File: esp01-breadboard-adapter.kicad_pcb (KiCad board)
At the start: 2 copper layers, 3 parts, among them P1 CONN_02X04, P2 CONN_01X04, P3 CONN_01X04

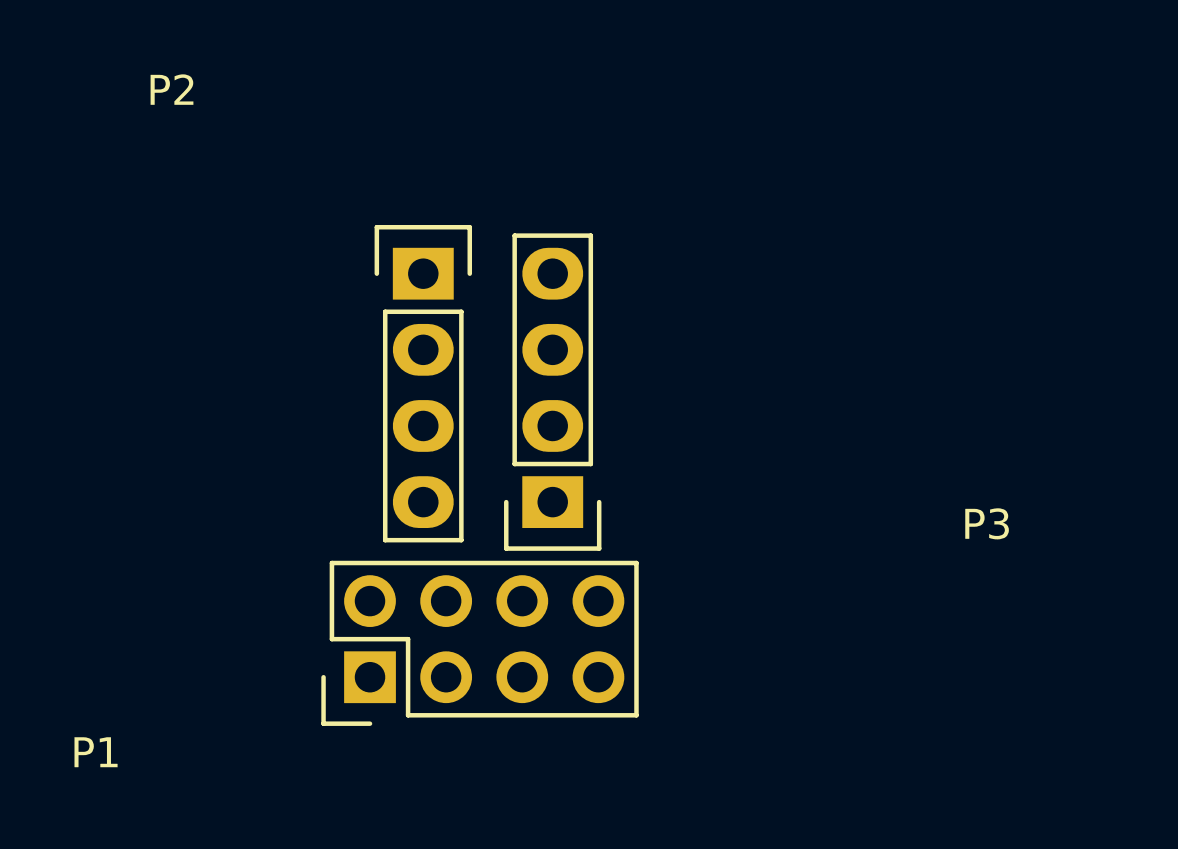
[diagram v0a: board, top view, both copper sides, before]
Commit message: begin 2nd layer pcb
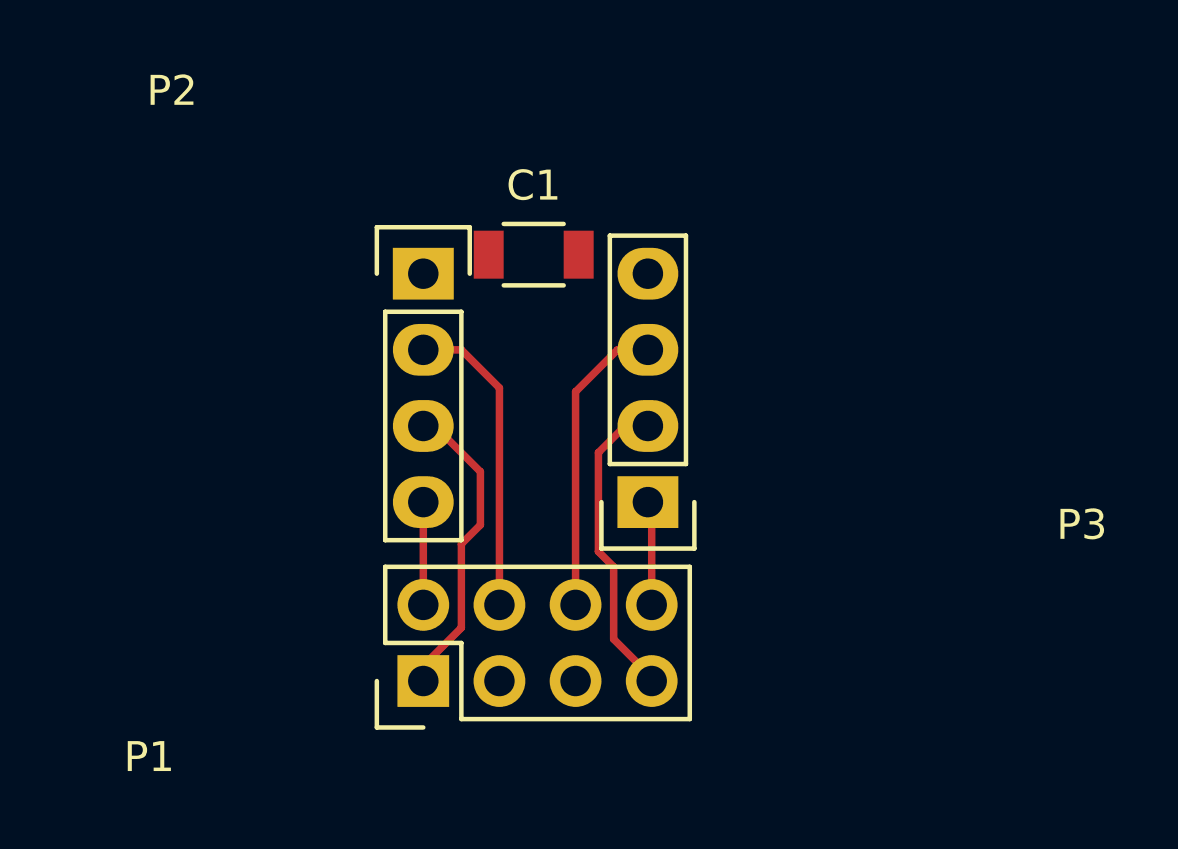
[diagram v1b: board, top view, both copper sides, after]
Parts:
- added C1: C, Capacitors_SMD:C_1206, F.Cu at (137.0, 106.6)
- moved P3 3.17 mm to (140.8, 114.8)
- moved P1 1.78 mm to (133.3, 120.8)
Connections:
- P2 pad 1: RXD -> GPIO0
- P2 pad 2: GPIO0 -> RESET
- P2 pad 3: GPIO2 -> RXD
- P2 pad 4: GND -> VCC
- P3 pad 2: CH_PD -> GND
- P3 pad 3: RESET -> CH_PD
- P3 pad 4: VCC -> GPIO2
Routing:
- net GND: track 0.00 -> 10.4 mm
- net RXD: track 0.00 -> 10.3 mm
- net RESET: track 0.00 -> 10.3 mm
- net CH_PD: track 0.00 -> 10.1 mm
- net TXD: track 0.00 -> 3.48 mm
- net VCC: track 0.00 -> 3.43 mm
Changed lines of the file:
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@@
 (kicad_pcb (version 4) (host pcbnew 4.0.2-stable)
   (general
-    (links 8)
-    (no_connects 8)
+    (links 10)
+    (no_connects 4)
     (area 0 0 0 0)
     (thickness 1.6)
     (drawings 0)
-    (tracks 0)
+    (tracks 23)
     (zones 0)
-    (modules 3)
+    (modules 4)
     (nets 9)
   )
@@
     (pad_to_mask_clearance 0.2)
     (aux_axis_origin 0 0)
-    (visible_elements FFFFFF7F)
+    (visible_elements 7FFFFFFF)
     (pcbplotparams
       (layerselection 0x00030_80000001)
@@
   )
   (module Pin_Headers:Pin_Header_Straight_2x04 (layer F.Cu)
-    (at 131.572 120.65 90)
+    (at 133.35 120.777 90)
     (descr "Through hole pin header")
     (tags "pin header")
@@
     (fp_line (start -1.55 -1.55) (end 1.55 -1.55) (layer F.SilkS) (width 0.15))
     (pad 1 thru_hole rect (at 0 0) (size 2.032 1.7272) (drill 1.016) (layers *.Cu *.Mask)
+      (net 3 GPIO0))
+    (pad 2 thru_hole oval (at 0 2.54) (size 2.032 1.7272) (drill 1.016) (layers *.Cu *.Mask)
+      (net 4 RESET))
+    (pad 3 thru_hole oval (at 0 5.08) (size 2.032 1.7272) (drill 1.016) (layers *.Cu *.Mask)
       (net 1 RXD))
-    (pad 2 thru_hole oval (at 0 2.54) (size 2.032 1.7272) (drill 1.016) (layers *.Cu *.Mask)
-      (net 3 GPIO0))
-    (pad 3 thru_hole oval (at 0 5.08) (size 2.032 1.7272) (drill 1.016) (layers *.Cu *.Mask)
-      (net 5 GPIO2))
     (pad 4 thru_hole oval (at 0 7.62) (size 2.032 1.7272) (drill 1.016) (layers *.Cu *.Mask)
-      (net 7 GND))
+      (net 2 VCC))
     (model Pin_Headers.3dshapes/Pin_Header_Straight_1x04.wrl
       (at (xyz 0 -0.15 0))
@@
   )
   (module Pin_Headers:Pin_Header_Straight_1x04 (layer F.Cu)
-    (at 137.668 114.808 180)
+    (at 140.843 114.808 180)
     (descr "Through hole pin header")
     (tags "pin header")
@@
       (net 8 TXD))
     (pad 2 thru_hole oval (at 0 2.54 180) (size 2.032 1.7272) (drill 1.016) (layers *.Cu *.Mask)
+      (net 7 GND))
+    (pad 3 thru_hole oval (at 0 5.08 180) (size 2.032 1.7272) (drill 1.016) (layers *.Cu *.Mask)
       (net 6 CH_PD))
-    (pad 3 thru_hole oval (at 0 5.08 180) (size 2.032 1.7272) (drill 1.016) (layers *.Cu *.Mask)
-      (net 4 RESET))
     (pad 4 thru_hole oval (at 0 7.62 180) (size 2.032 1.7272) (drill 1.016) (layers *.Cu *.Mask)
-      (net 2 VCC))
+      (net 5 GPIO2))
     (model Pin_Headers.3dshapes/Pin_Header_Straight_1x04.wrl
       (at (xyz 0 -0.15 0))
@@
     )
   )
+  (module Capacitors_SMD:C_1206 (layer F.Cu)
+    (at 137.033 106.553)
+    (descr "Capacitor SMD 1206, reflow soldering, AVX (see smccp.pdf)")
+    (tags "capacitor 1206")
+    (attr smd)
+    (fp_text reference C1 (at 0 -2.3) (layer F.SilkS)
+      (effects (font (size 1 1) (thickness 0.15)))
+    )
+    (fp_text value C (at 0 2.3) (layer F.Fab)
+      (effects (font (size 1 1) (thickness 0.15)))
+    )
+    (fp_line (start -1.6 0.8) (end -1.6 -0.8) (layer F.Fab) (width 0.15))
+    (fp_line (start 1.6 0.8) (end -1.6 0.8) (layer F.Fab) (width 0.15))
+    (fp_line (start 1.6 -0.8) (end 1.6 0.8) (layer F.Fab) (width 0.15))
+    (fp_line (start -1.6 -0.8) (end 1.6 -0.8) (layer F.Fab) (width 0.15))
+    (fp_line (start -2.3 -1.15) (end 2.3 -1.15) (layer F.CrtYd) (width 0.05))
+    (fp_line (start -2.3 1.15) (end 2.3 1.15) (layer F.CrtYd) (width 0.05))
+    (fp_line (start -2.3 -1.15) (end -2.3 1.15) (layer F.CrtYd) (width 0.05))
+    (fp_line (start 2.3 -1.15) (end 2.3 1.15) (layer F.CrtYd) (width 0.05))
+    (fp_line (start 1 -1.025) (end -1 -1.025) (layer F.SilkS) (width 0.15))
+    (fp_line (start -1 1.025) (end 1 1.025) (layer F.SilkS) (width 0.15))
+    (pad 1 smd rect (at -1.5 0) (size 1 1.6) (layers F.Cu F.Paste F.Mask)
+      (net 2 VCC))
+    (pad 2 smd rect (at 1.5 0) (size 1 1.6) (layers F.Cu F.Paste F.Mask)
+      (net 7 GND))
+    (model Capacitors_SMD.3dshapes/C_1206.wrl
+      (at (xyz 0 0 0))
+      (scale (xyz 1 1 1))
+      (rotate (xyz 0 0 0))
+    )
+  )
+  (segment (start 133.35 120.777) (end 133.35 120.269) (width 0.25) (layer F.Cu) (net 1) (status C00000))
+  (segment (start 133.35 120.269) (end 134.62 118.999) (width 0.25) (layer F.Cu) (net 1) (status 400000))
+  (segment (start 134.62 118.999) (end 134.62 116.205) (width 0.25) (layer F.Cu) (net 1))
+  (segment (start 134.62 116.205) (end 135.255 115.57) (width 0.25) (layer F.Cu) (net 1))
+  (segment (start 135.255 115.57) (end 135.255 113.792) (width 0.25) (layer F.Cu) (net 1))
+  (segment (start 135.255 113.792) (end 133.731 112.268) (width 0.25) (layer F.Cu) (net 1) (status 800000))
+  (segment (start 133.731 112.268) (end 133.35 112.268) (width 0.25) (layer F.Cu) (net 1) (status C00000))
+  (segment (start 133.35 118.237) (end 133.35 114.808) (width 0.25) (layer F.Cu) (net 2))
+  (segment (start 135.89 118.237) (end 135.89 110.998) (width 0.25) (layer F.Cu) (net 4))
+  (segment (start 134.62 109.728) (end 133.35 109.728) (width 0.25) (layer F.Cu) (net 4))
+  (segment (start 135.89 110.998) (end 134.62 109.728) (width 0.25) (layer F.Cu) (net 4))
+  (segment (start 138.43 118.237) (end 138.43 111.125) (width 0.25) (layer F.Cu) (net 6))
+  (segment (start 138.43 111.125) (end 139.827 109.728) (width 0.25) (layer F.Cu) (net 6))
+  (segment (start 139.827 109.728) (end 140.843 109.728) (width 0.25) (layer F.Cu) (net 6))
+  (segment (start 140.97 120.777) (end 140.97 120.65) (width 0.25) (layer F.Cu) (net 7) (status C00000))
+  (segment (start 140.97 120.65) (end 139.7 119.38) (width 0.25) (layer F.Cu) (net 7) (status 400000))
+  (segment (start 139.7 119.38) (end 139.7 116.967) (width 0.25) (layer F.Cu) (net 7))
+  (segment (start 139.7 116.967) (end 139.192 116.459) (width 0.25) (layer F.Cu) (net 7))
+  (segment (start 139.192 116.459) (end 139.192 113.157) (width 0.25) (layer F.Cu) (net 7))
+  (segment (start 139.192 113.157) (end 140.081 112.268) (width 0.25) (layer F.Cu) (net 7) (status 800000))
+  (segment (start 140.081 112.268) (end 140.843 112.268) (width 0.25) (layer F.Cu) (net 7) (status C00000))
+  (segment (start 140.97 118.237) (end 140.97 114.935) (width 0.25) (layer F.Cu) (net 8))
+  (segment (start 140.97 114.935) (end 140.843 114.808) (width 0.25) (layer F.Cu) (net 8))
 )
